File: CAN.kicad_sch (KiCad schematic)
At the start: 5 parts, among them U501 U_SIT1044TK/3

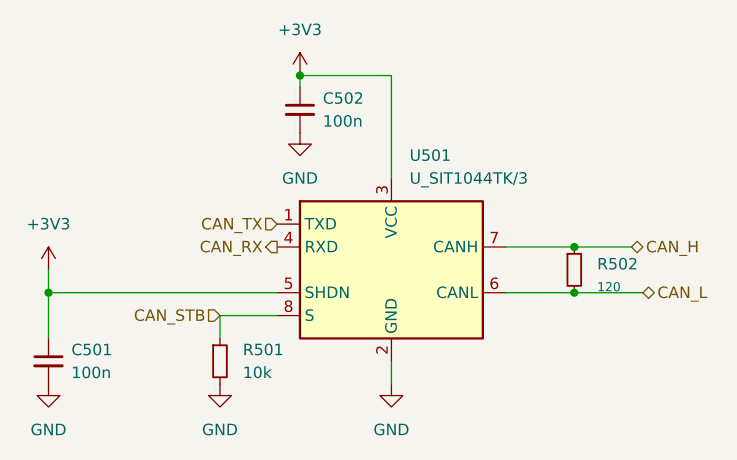
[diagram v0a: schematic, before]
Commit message: layout: finalize most of the layout
Signed-off-by: Connor Rigby <connorr@hey.com>
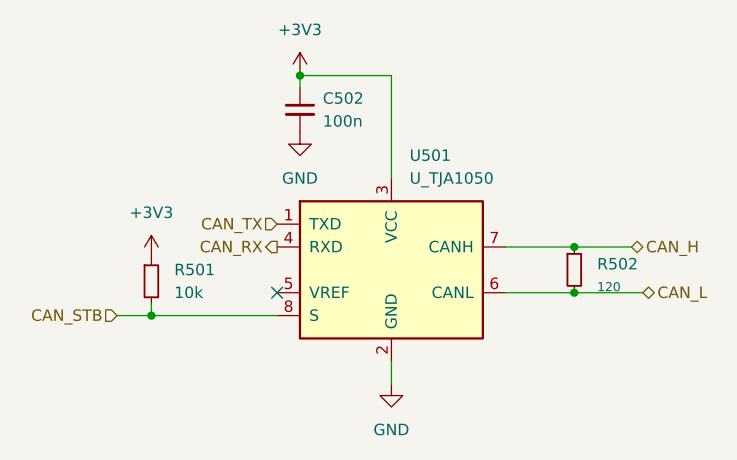
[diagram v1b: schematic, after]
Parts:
- removed C501: C_0402_100n, Capacitor_SMD:C_0402_1005Metric, symbol BOM:C_0402_100n
- removed U501: U_SIT1044TK/3, Package_SON:HVSON-8-1EP_3x3mm_P0.65mm_EP1.6x2.4mm, symbol BOM:U_SIT1044TK/3
- added U501: U_TJA1050, Package_SO:SOIC-8_3.9x4.9mm_P1.27mm, symbol BOM:U_TJA1050
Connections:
- net +3V3: now also R501.1, U501.3 (VCC)
- net CAN_H: now also U501.7 (CANH)
- net CAN_L: now also U501.6 (CANL)
- net CAN_RX: now also U501.4 (RXD)
- net CAN_STB: now also R501.2, U501.8 (S); no longer R501.1
- net CAN_TX: now also U501.1 (TXD)
- net GND: now also U501.2 (GND); no longer R501.2
- no-connect marks 0 -> 1
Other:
- moved on the sheet: R501
